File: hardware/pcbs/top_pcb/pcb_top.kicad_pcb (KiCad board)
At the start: 2 copper layers, 105 x 47 mm, 20 parts, among them J1 molex1x03, U1 ATtiny1626, U2 74hc4066, U3 74hc4066, U4 74hc4066, U5 74hc4066, U6 74hc4066, U7 74hc4066, U8 74hc4066, U9 74hc4066

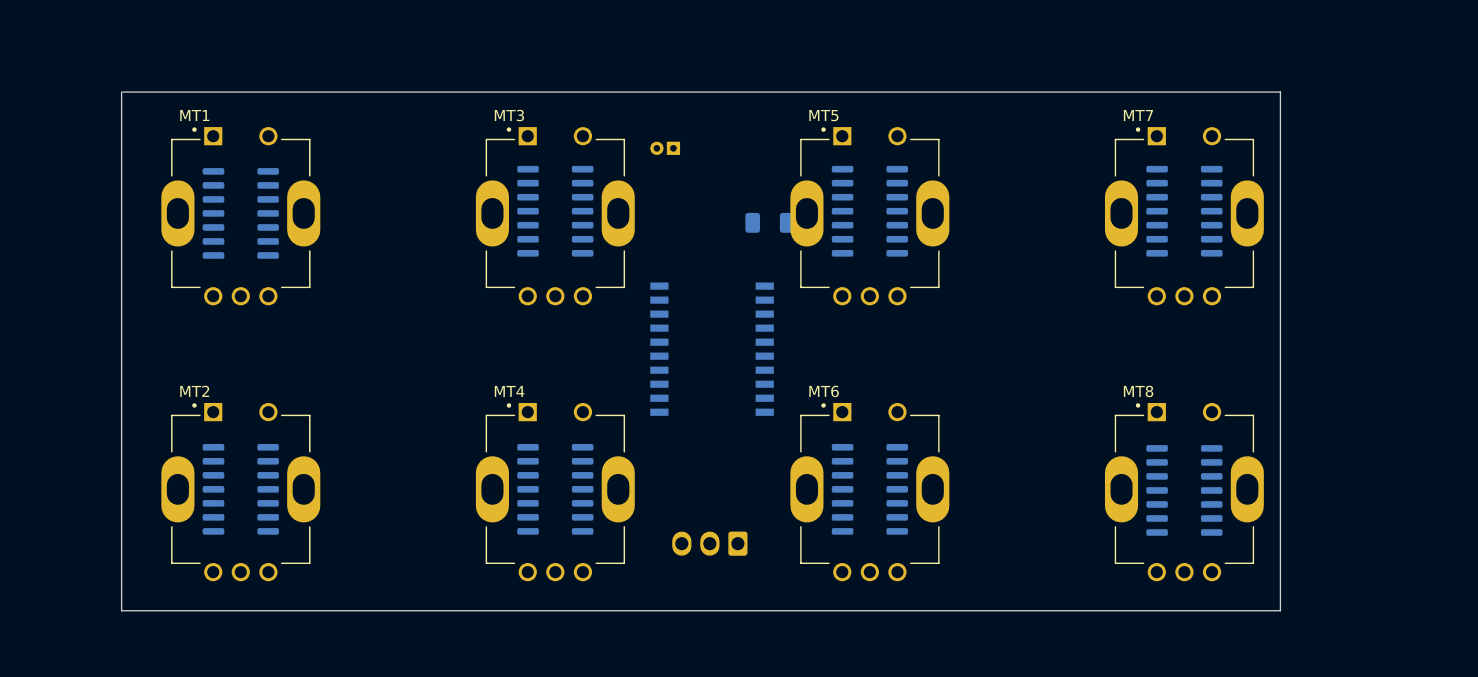
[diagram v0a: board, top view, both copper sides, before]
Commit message: ,,
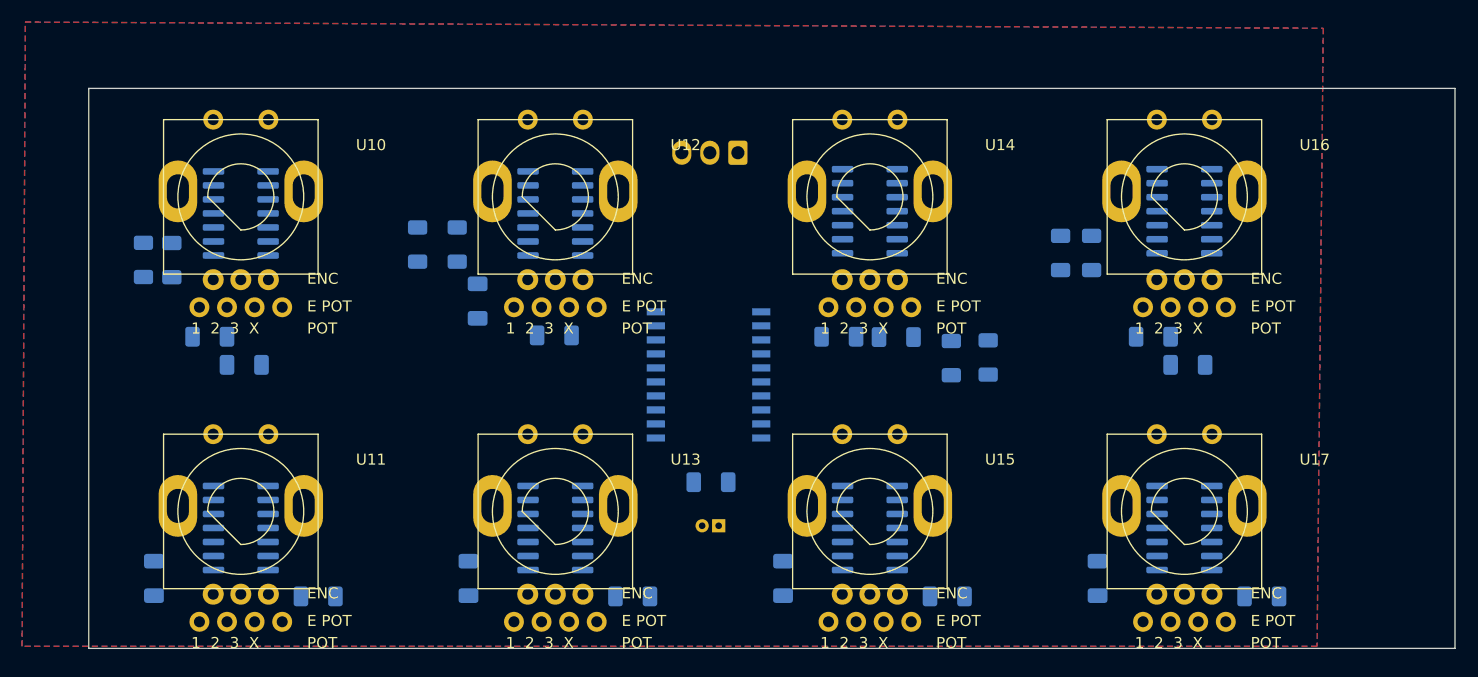
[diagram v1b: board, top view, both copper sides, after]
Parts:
- removed MT1, MT2, MT3, MT4, MT5, MT6, MT7, MT8: PEC11R-4215F-S0024, 3dAudioFoot:XDCR_PEC11R-4215F-S0024
- added C10: 100n, Capacitor_SMD:C_1206_3216Metric_Pad1.33x1.80mm_HandSolder, B.Cu at (101.3, 83.7)
- added C11: 100n, Capacitor_SMD:C_1206_3216Metric_Pad1.33x1.80mm_HandSolder, B.Cu at (120.0, 60.2)
- added C12: 100n, Capacitor_SMD:C_1206_3216Metric_Pad1.33x1.80mm_HandSolder, B.Cu at (114.9, 82.1)
- added C13: 100n, Capacitor_SMD:C_1206_3216Metric_Pad1.33x1.80mm_HandSolder, B.Cu at (125.2, 60.2)
- added C14: 100n, Capacitor_SMD:C_1206_3216Metric_Pad1.33x1.80mm_HandSolder, B.Cu at (129.8, 83.7)
- added C15: 100n, Capacitor_SMD:C_1206_3216Metric_Pad1.33x1.80mm_HandSolder, B.Cu at (148.5, 60.2)
- added C16: 100n, Capacitor_SMD:C_1206_3216Metric_Pad1.33x1.80mm_HandSolder, B.Cu at (143.4, 82.1)
- added C17: 100n, Capacitor_SMD:C_1206_3216Metric_Pad1.33x1.80mm_HandSolder, B.Cu at (151.6, 62.7)
- added C18: 100n, Capacitor_SMD:C_1206_3216Metric_Pad1.33x1.80mm_HandSolder, B.Cu at (158.3, 83.7)
- added C3: 100n, Capacitor_SMD:C_1206_3216Metric_Pad1.33x1.80mm_HandSolder, B.Cu at (63.0, 60.2)
- added C4: 100n, Capacitor_SMD:C_1206_3216Metric_Pad1.33x1.80mm_HandSolder, B.Cu at (66.1, 62.7)
- added C5: 100n, Capacitor_SMD:C_1206_3216Metric_Pad1.33x1.80mm_HandSolder, B.Cu at (57.9, 82.1)
- added C6: 100n, Capacitor_SMD:C_1206_3216Metric_Pad1.33x1.80mm_HandSolder, B.Cu at (72.8, 83.7)
- added C7: 100n, Capacitor_SMD:C_1206_3216Metric_Pad1.33x1.80mm_HandSolder, B.Cu at (87.3, 56.9)
- added C8: 100n, Capacitor_SMD:C_1206_3216Metric_Pad1.33x1.80mm_HandSolder, B.Cu at (86.4, 82.1)
- added C9: 100n, Capacitor_SMD:C_1206_3216Metric_Pad1.33x1.80mm_HandSolder, B.Cu at (94.2, 60.0)
- added R25: 10k, Resistor_SMD:R_1206_3216Metric_Pad1.30x1.75mm_HandSolder, B.Cu at (85.4, 51.8)
- added R26: 10k, Resistor_SMD:R_1206_3216Metric_Pad1.30x1.75mm_HandSolder, B.Cu at (133.5, 62.0)
- added R27: 10k, Resistor_SMD:R_1206_3216Metric_Pad1.30x1.75mm_HandSolder, B.Cu at (142.9, 52.6)
- added R28: 10k, Resistor_SMD:R_1206_3216Metric_Pad1.30x1.75mm_HandSolder, B.Cu at (57.0, 53.2)
- added R29: 10k, Resistor_SMD:R_1206_3216Metric_Pad1.30x1.75mm_HandSolder, B.Cu at (81.8, 51.8)
- added R3: 10k, Resistor_SMD:R_1206_3216Metric_Pad1.30x1.75mm_HandSolder, B.Cu at (59.5, 53.2)
- added R30: 10k, Resistor_SMD:R_1206_3216Metric_Pad1.30x1.75mm_HandSolder, B.Cu at (130.2, 62.1)
- added R31: 10k, Resistor_SMD:R_1206_3216Metric_Pad1.30x1.75mm_HandSolder, B.Cu at (140.1, 52.6)
- added U10: ~, 3dAudioFoot:Encoder und Endless, F.Cu at (65.8, 47.5)
- added U11: ~, 3dAudioFoot:Encoder und Endless, F.Cu at (65.8, 76.0)
- added U12: ~, 3dAudioFoot:Encoder und Endless, F.Cu at (94.3, 47.5)
- added U13: ~, 3dAudioFoot:Encoder und Endless, F.Cu at (94.3, 76.0)
- added U14: ~, 3dAudioFoot:Encoder und Endless, F.Cu at (122.8, 47.5)
- added U15: ~, 3dAudioFoot:Encoder und Endless, F.Cu at (122.8, 76.0)
- added U16: ~, 3dAudioFoot:Encoder und Endless, F.Cu at (151.3, 47.5)
- added U17: ~, 3dAudioFoot:Encoder und Endless, F.Cu at (151.3, 76.0)
- moved J1 35.4 mm to (110.8, 43.5)
- moved C1 34.4 mm to (109.1, 77.3)
- moved C2 24.1 mm to (108.4, 73.3)
- moved U3 3.50 mm to (65.8, 77.5), turned to 0 degrees
- moved U5 3.50 mm to (94.3, 77.5), turned to 0 degrees
- moved U7 3.50 mm to (122.8, 77.5), turned to 0 degrees
- moved U9 3.40 mm to (151.3, 77.5), turned to 0 degrees
- moved U1 2.35 mm to (108.2, 63.6), turned to 0 degrees
- moved U4 0.20 mm to (94.3, 49.0), turned to 0 degrees
- turned U2 to 0 degrees
- turned U6 to 0 degrees
- turned U8 to 0 degrees
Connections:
- U3 pad 9: /Untitled Sheet/ENC_A_SW -> /Untitled Sheet/ENC_B_SW
- U4 pad 9: /Untitled Sheet/ENC_B_SW -> /Untitled Sheet/ENC_A_SW
- U7 pad 9: /Untitled Sheet/ENC_C_SW -> /Untitled Sheet/ENC_D_SW
- U8 pad 9: /Untitled Sheet/ENC_D_SW -> /Untitled Sheet/ENC_C_SW
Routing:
- added copper zone on B.Cu, net GND
- added copper zone on F.Cu, net GND
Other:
- board size 105 x 47 mm -> 123.8 x 50.7 mm
